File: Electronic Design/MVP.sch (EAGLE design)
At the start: 38 parts, among them IC1 ACS711KLCTR-12AB-T, IC3 ATMEGA328-PU, Q2 16MHz, Q3 IRF9540, Q4 IRF9540

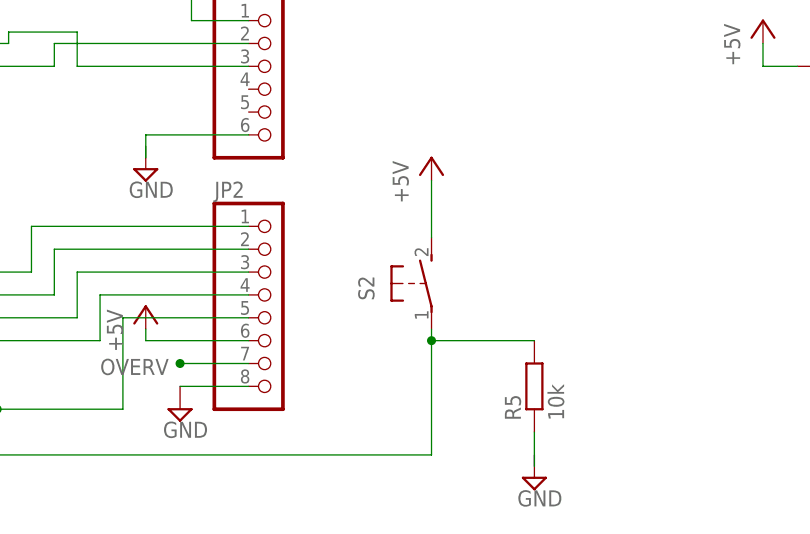
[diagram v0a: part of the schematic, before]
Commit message: First pass at adding traces
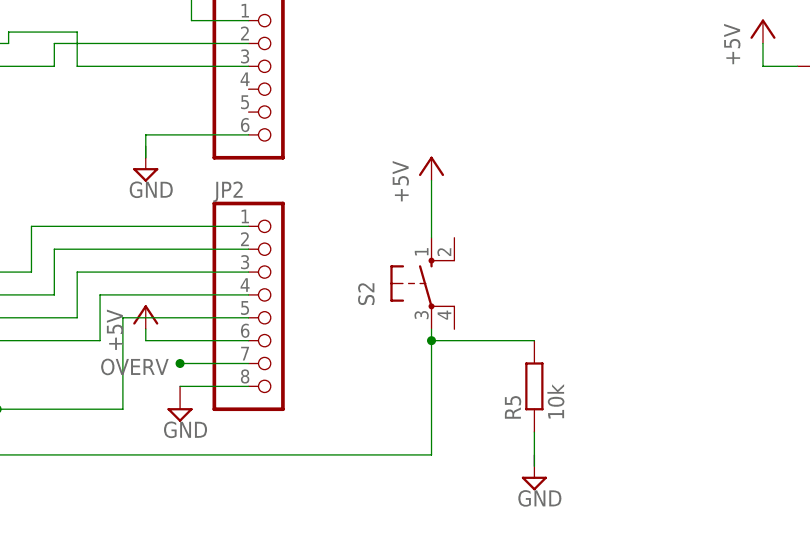
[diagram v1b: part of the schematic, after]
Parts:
- S2: device switch-omron:31-XX -> switch-omron:10-XX
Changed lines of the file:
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@@
 <setting verticaltext="up"/>
 </settings>
-<grid distance="0.05" unitdist="inch" unit="inch" style="lines" multiple="1" display="no" altdistance="0.01" altunitdist="inch" altunit="inch"/>
+<grid distance="0.1" unitdist="inch" unit="inch" style="lines" multiple="1" display="no" altdistance="0.01" altunitdist="inch" altunit="inch"/>
 <layers>
 <layer number="1" name="Top" color="4" fill="1" visible="no" active="no"/>
@@
 <part name="S1" library="switch" deviceset="255SB" device=""/>
 <part name="USB_OUT" library="pinhead" deviceset="PINHD-1X3" device=""/>
-<part name="S2" library="switch-omron" deviceset="31-XX" device=""/>
+<part name="S2" library="switch-omron" deviceset="10-XX" device=""/>
 <part name="+5V2" library="supply1" deviceset="+5V" device=""/>
 <part name="R5" library="resistor" deviceset="R-EU_" device="R1210" value="10k"/>
